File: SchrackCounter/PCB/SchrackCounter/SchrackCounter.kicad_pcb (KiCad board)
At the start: 4 copper layers, 100 x 65 mm, 59 parts, among them IC1 TPS565242DRLR, J1 TYPE-C-31-M-12, J2 Conn_01x02_Pin, J3 Conn_01x02_Pin, M1 Fan_CPU_4pin, SW1 SW_DPDT_x2, SW2 SW_Push, SW3 SW_Push, SW4 SW_Push, SW5 SW_Push, SW6 SW_Push, SW7 SW_Push, SW8 SW_Push, U1 LTD080BUE-103A, U2 LTD080BUE-103A, U3 LTD080BUE-103A, U6 MAX7219, U7 ESP32-S3-WROOM-2, U8 USBLC6-2SC6

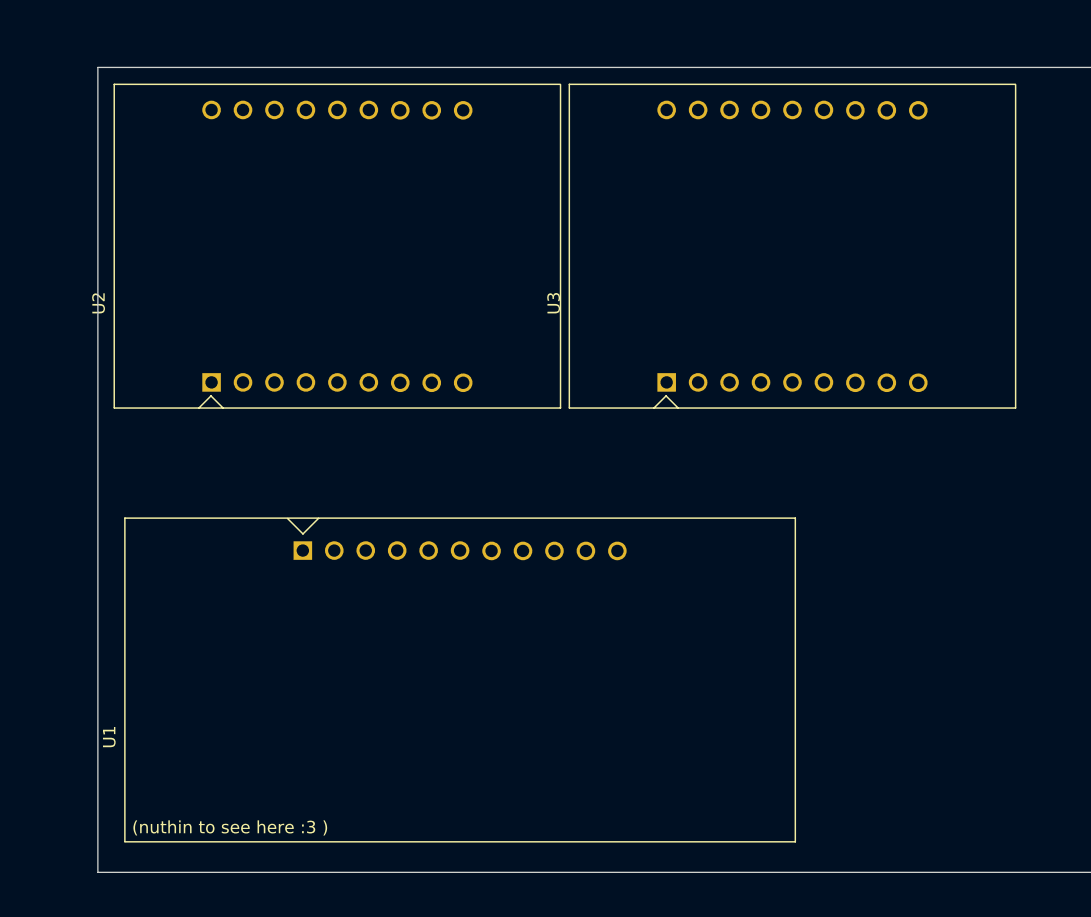
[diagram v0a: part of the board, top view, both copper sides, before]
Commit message: Im doing 3d models now i guess
New 3digit and 2digit 3d models, kinda proud of them even tho im committed 5 warcrimes while making them
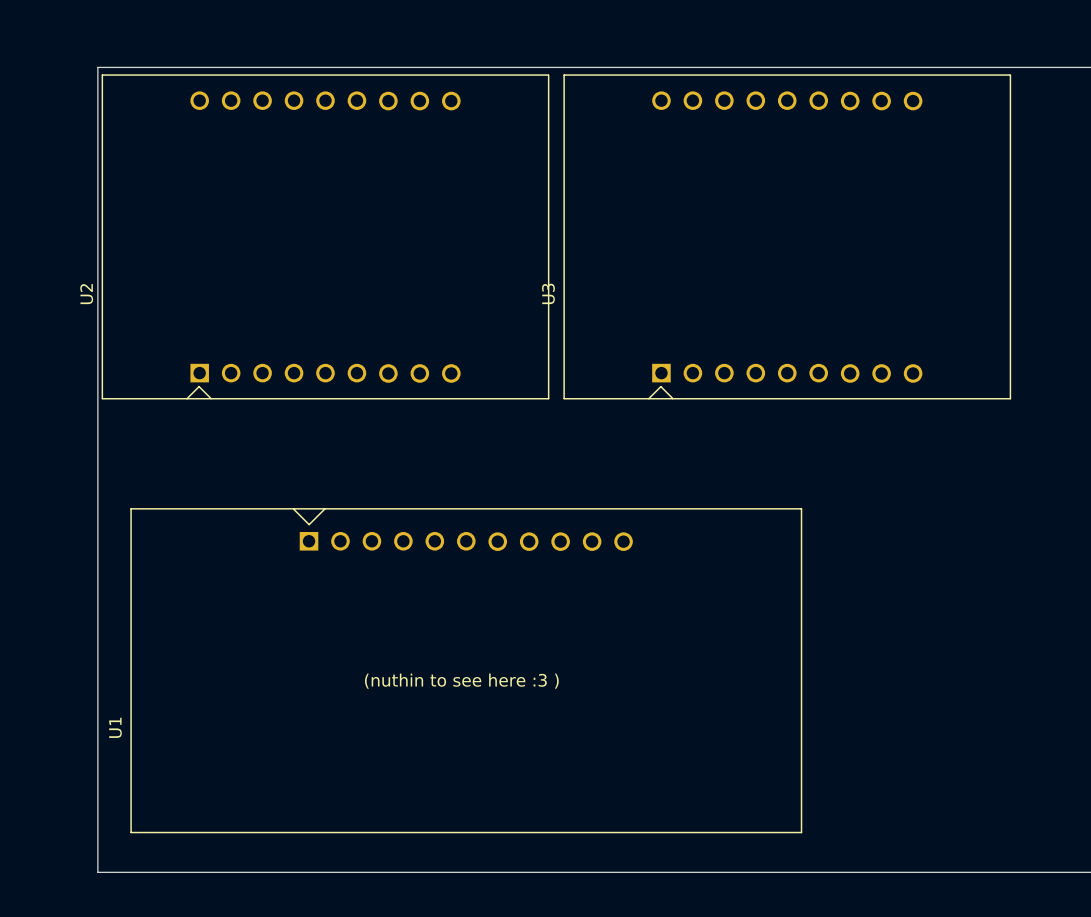
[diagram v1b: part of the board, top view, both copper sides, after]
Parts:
- moved U2 1.22 mm to (65.7, 70.2)
- moved U1 0.90 mm to (68.0, 105.2)
- moved U3 0.86 mm to (103.0, 70.2)
